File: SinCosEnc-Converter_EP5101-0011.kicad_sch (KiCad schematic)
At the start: 39 parts, among them J1 Conn_01x05_Pin, J2 Conn_02x05_Top_Bottom, SW1 SW_RCLK, SW2 SW_SG1, SW3 SW_SG0, SW4 SW_ROT, SW5 SW_SF1, SW6 SW_SF0, U1 iC-NV, X2 D-SUB-DR-15PCG-AB

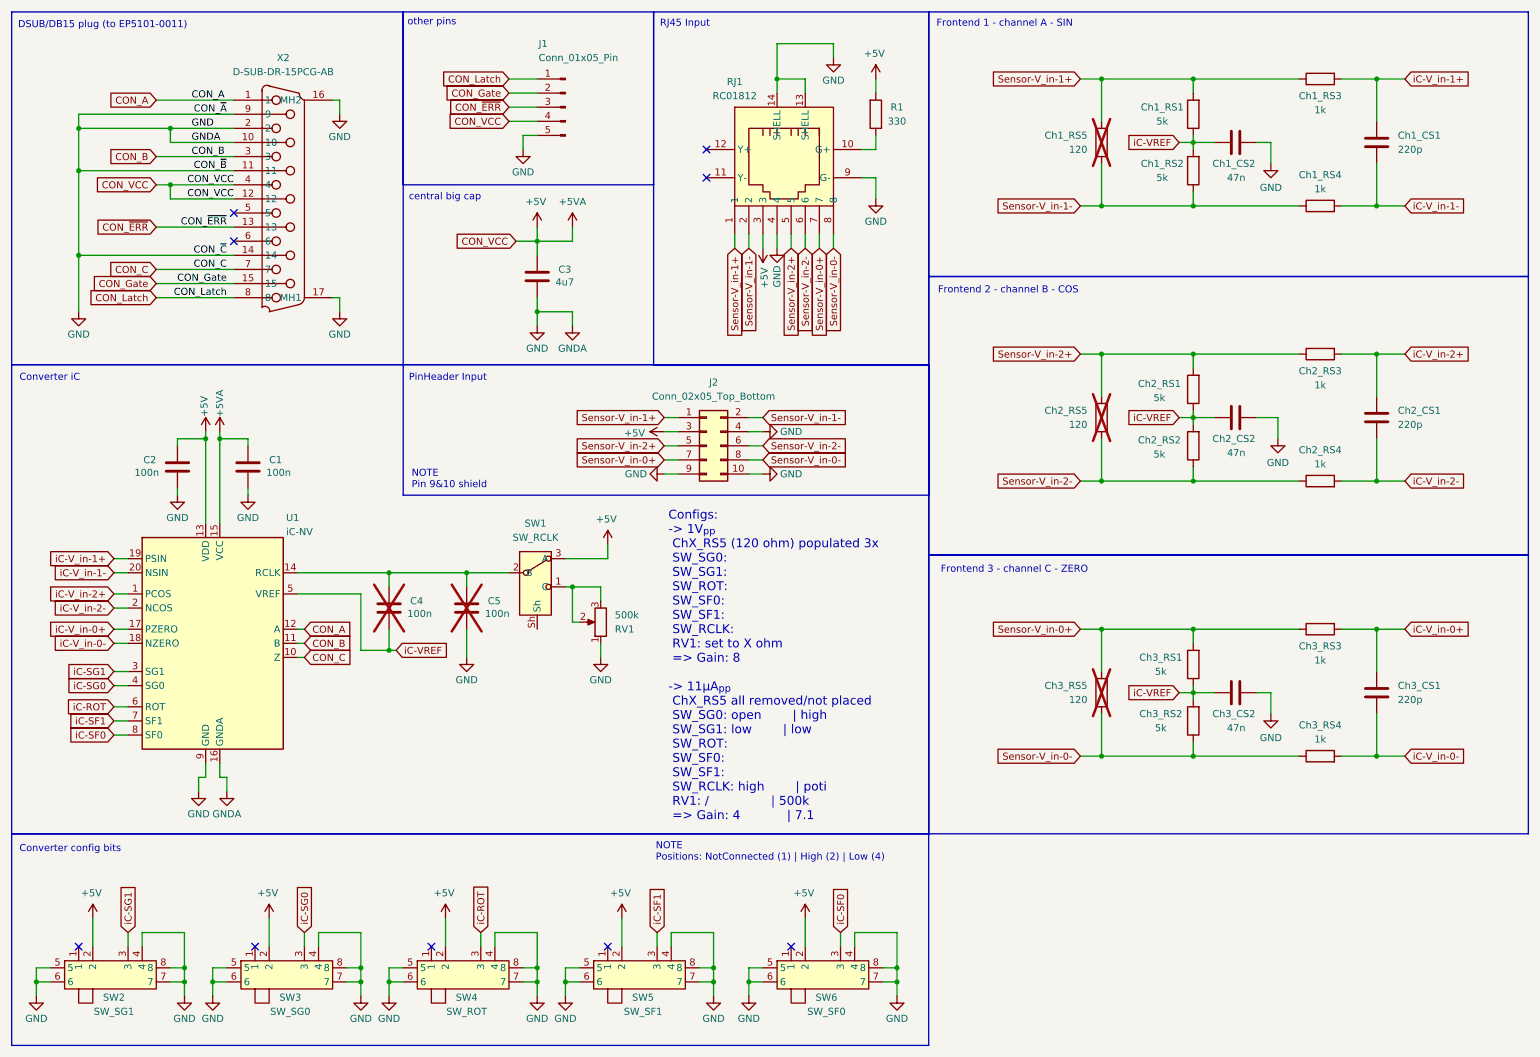
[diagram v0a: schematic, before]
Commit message: finished schematics for v0.9.0, PCB ToDo
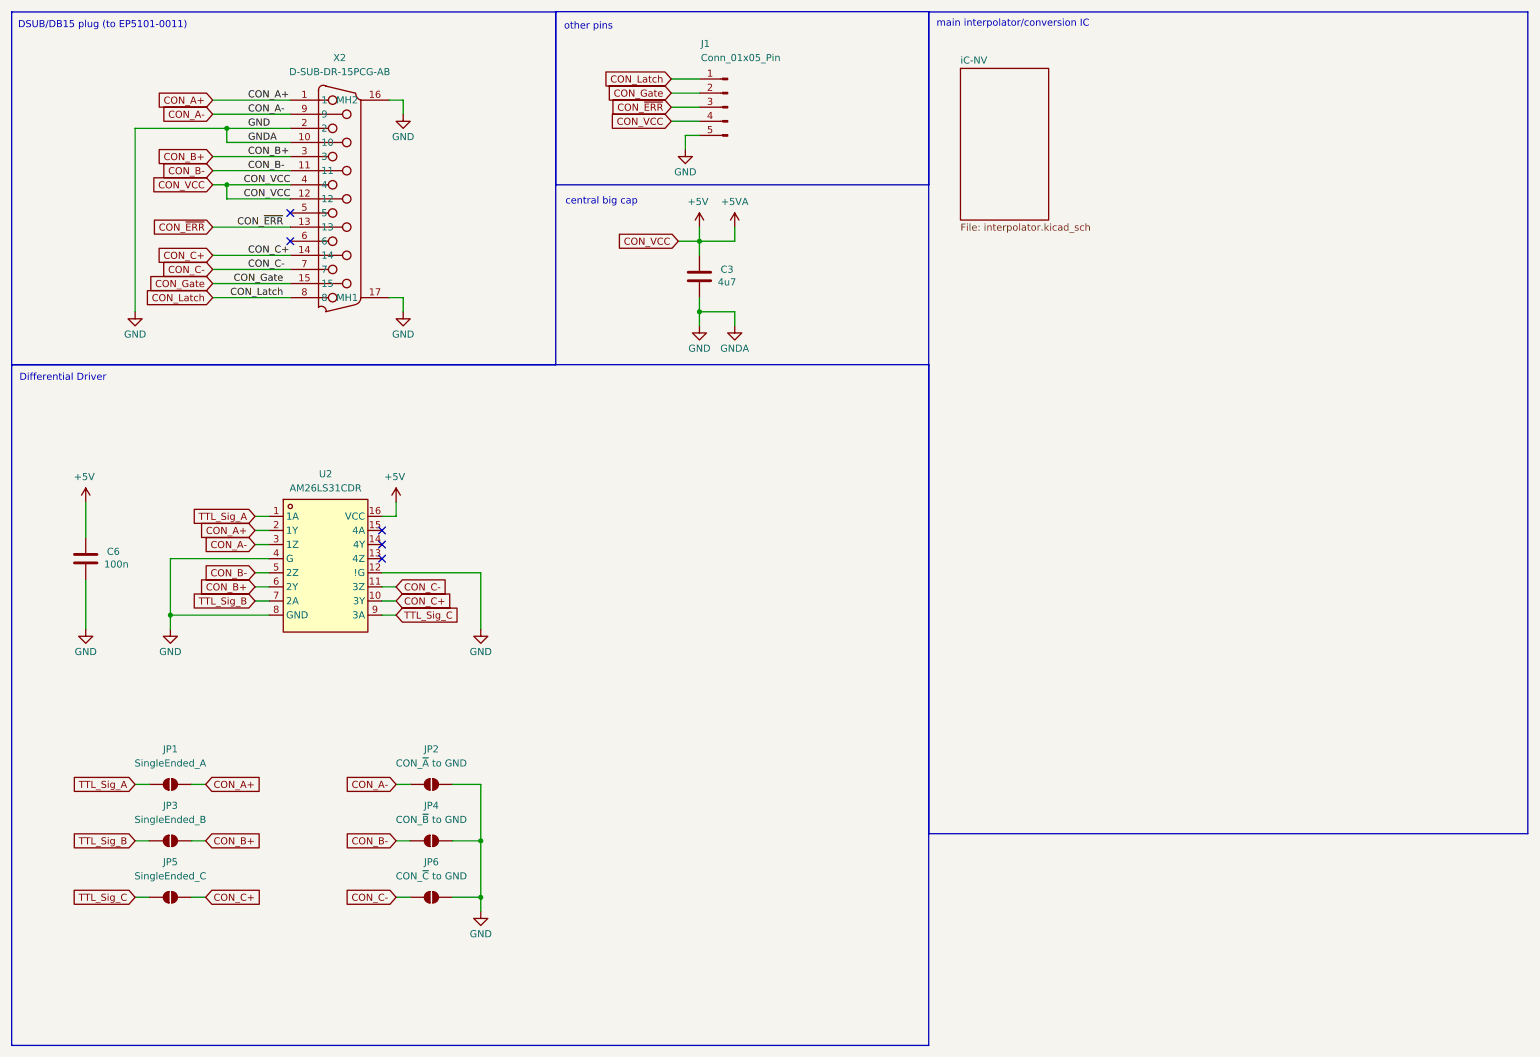
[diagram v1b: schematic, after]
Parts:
- removed C1, C2, C4, C5: 100n, Capacitor_SMD:C_0603_1608Metric, symbol Device:C
- removed Ch1_CS1, Ch2_CS1, Ch3_CS1: 220p, Capacitor_SMD:C_0603_1608Metric, symbol Device:C
- removed Ch1_CS2, Ch2_CS2, Ch3_CS2: 47n, Capacitor_SMD:C_0603_1608Metric, symbol Device:C
- removed Ch1_RS1, Ch1_RS2, Ch2_RS1, Ch2_RS2, Ch3_RS1, Ch3_RS2: 5k, Resistor_SMD:R_0603_1608Metric, symbol Device:R
- removed Ch1_RS3, Ch1_RS4, Ch2_RS3, Ch2_RS4, Ch3_RS3, Ch3_RS4: 1k, Resistor_SMD:R_0603_1608Metric, symbol Device:R
- removed Ch1_RS5, Ch2_RS5, Ch3_RS5: 120, Resistor_SMD:R_0603_1608Metric, symbol Device:R
- removed J2: Conn_02x05_Top_Bottom, Connector_PinHeader_2.54mm:PinHeader_2x05_P2.54mm_Horizontal, symbol Connector_Generic:Conn_02x05_Odd_Even
- removed R1: 330, Resistor_SMD:R_0603_1608Metric, symbol Device:R
- removed RJ1: RC01812, easyeda2kicad:RJ45-TH_RC01812, symbol easyeda2kicad:RC01812
- removed RV1: 500k, Potentiometer_THT:Potentiometer_Bourns_3296P_Horizontal, symbol Device:R_Potentiometer
- removed SW1: SW_RCLK, CostumLibrary:SW-SMD_XKB_SS-3292S-L2-W, symbol CostumLibrary:SS-3292S-L2-W
- removed SW2: SW_SG1, easyeda2kicad:SW-SMD_MSK13C02-BB, symbol easyeda2kicad:HXMSK13C02
- removed SW3: SW_SG0, easyeda2kicad:SW-SMD_MSK13C02-BB, symbol easyeda2kicad:HXMSK13C02
- removed SW4: SW_ROT, easyeda2kicad:SW-SMD_MSK13C02-BB, symbol easyeda2kicad:HXMSK13C02
- removed SW5: SW_SF1, easyeda2kicad:SW-SMD_MSK13C02-BB, symbol easyeda2kicad:HXMSK13C02
- removed SW6: SW_SF0, easyeda2kicad:SW-SMD_MSK13C02-BB, symbol easyeda2kicad:HXMSK13C02
- removed U1: iC-NV, Package_SO:TSSOP-20_4.4x6.5mm_P0.65mm, symbol CostumLibrary:iC-NV
- added C6: 100n, Capacitor_SMD:C_0603_1608Metric, symbol Device:C
- added JP1: SingleEnded_A, Jumper:SolderJumper-2_P1.3mm_Open_RoundedPad1.0x1.5mm, symbol Jumper:SolderJumper_2_Open
- added JP2: CON_~{A} to GND, Jumper:SolderJumper-2_P1.3mm_Open_RoundedPad1.0x1.5mm, symbol Jumper:SolderJumper_2_Open
- added JP3: SingleEnded_B, Jumper:SolderJumper-2_P1.3mm_Open_RoundedPad1.0x1.5mm, symbol Jumper:SolderJumper_2_Open
- added JP4: CON_~{B} to GND, Jumper:SolderJumper-2_P1.3mm_Open_RoundedPad1.0x1.5mm, symbol Jumper:SolderJumper_2_Open
- added JP5: SingleEnded_C, Jumper:SolderJumper-2_P1.3mm_Open_RoundedPad1.0x1.5mm, symbol Jumper:SolderJumper_2_Open
- added JP6: CON_~{C} to GND, Jumper:SolderJumper-2_P1.3mm_Open_RoundedPad1.0x1.5mm, symbol Jumper:SolderJumper_2_Open
- added U2: AM26LS31CDR, easyeda2kicad:SOIC-16_L9.9-W3.9-P1.27-LS6.0-BL, symbol easyeda2kicad:AM26LS31CDR
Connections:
- net +5V: now also C6.2, U2.16 (VCC)
- net GND: now also C6.1, JP2.2 (B), JP4.2 (B), JP6.2 (B), U2.12 (!G), U2.4 (G), U2.8 (GND); no longer X2.11, X2.14, X2.9
- net CON_A renamed CON_A+
- net CON_A+: now also JP1.2 (B), U2.2 (1Y)
- net CON_B renamed CON_B+
- net CON_B+: now also JP3.2 (B), U2.6 (2Y)
- net CON_C renamed CON_C-
- net CON_C-: now also JP6.1 (A), U2.11 (3Z)
- new net CON_A-: JP2.1 (A), U2.3 (1Z), X2.9
- new net CON_B-: JP4.1 (A), U2.5 (2Z), X2.11
- new net CON_C+: JP5.2 (B), U2.10 (3Y), X2.14
- new net TTL_Sig_A: JP1.1 (A), U2.1 (1A)
- new net TTL_Sig_B: JP3.1 (A), U2.7 (2A)
- new net TTL_Sig_C: JP5.1 (A), U2.9 (3A)
- no-connect marks 9 -> 5
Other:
- added sheet iC-NV (interpolator.kicad_sch)
- note added: "Differential Driver"
- note added: "main interpolator/conversion IC"
- note removed: "Configs: -> 1V_{pp} ChX_RS5 (120 ohm) populated 3x SW_SG0: SW_SG1: SW_ROT: SW_SF0: SW_SF1: SW_RCLK: RV1: set to X ohm => Gain: 8 -> 11µA_{pp} ChX_RS5 all removed/not placed SW_SG0: open | high SW_SG1: low | low SW_ROT: SW_SF0: SW_SF1: SW_RCLK: high | poti RV1: / | 500k => Gain: 4 | 7.1"
- note removed: "Converter config bits"
- note removed: "Converter iC"
- note removed: "Frontend 1 - channel A - SIN"
- note removed: "Frontend 2 - channel B - COS"
- note removed: "Frontend 3 - channel C - ZERO"
- note removed: "NOTE Pin 9&10 shield"
- note removed: "NOTE Positions: NotConnected (1) | High (2) | Low (4)"
- note removed: "PinHeader Input"
- note removed: "RJ45 Input"
- title: (none) -> Header and Outputs
- moved on the sheet: C3, J1, X2
